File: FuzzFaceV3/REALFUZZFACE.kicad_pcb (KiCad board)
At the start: 2 copper layers, 48.5 x 35.2 mm, 22 parts, among them Q1 2SA1015, Q2 2SA1015

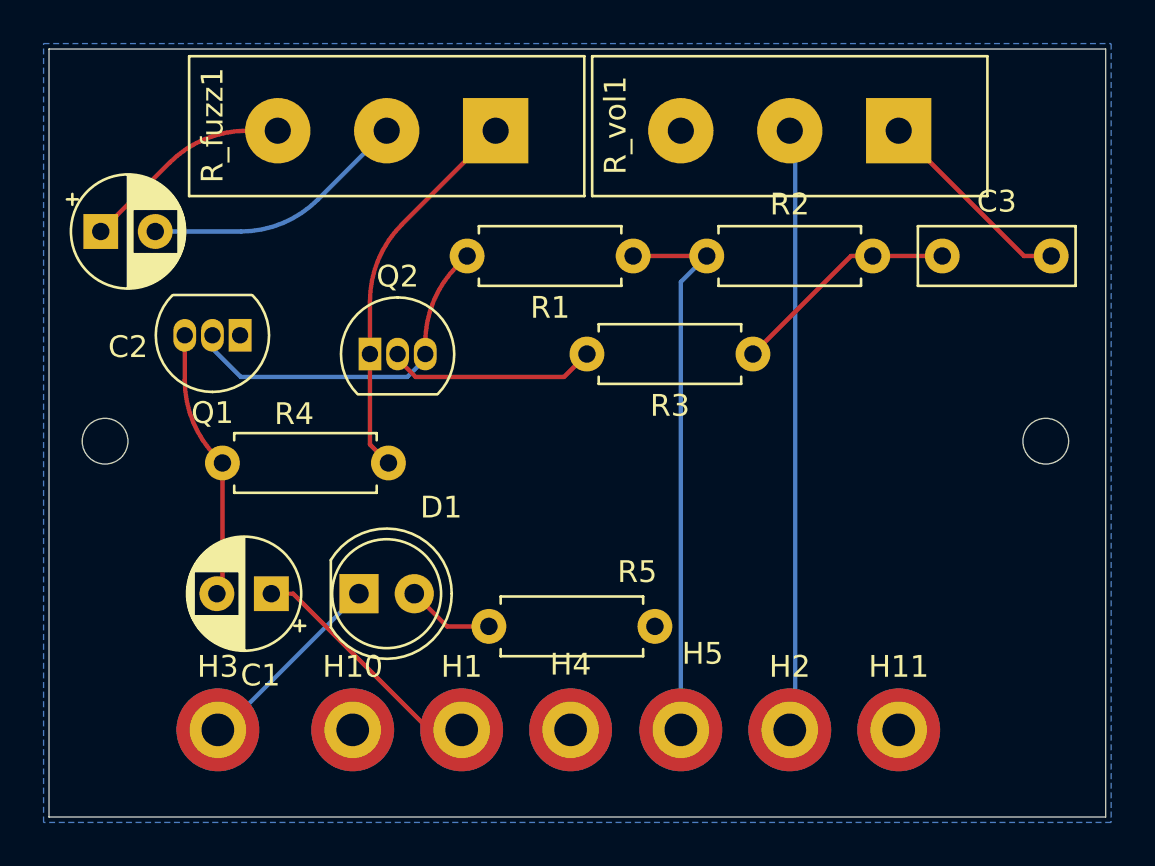
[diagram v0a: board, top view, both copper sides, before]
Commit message: done
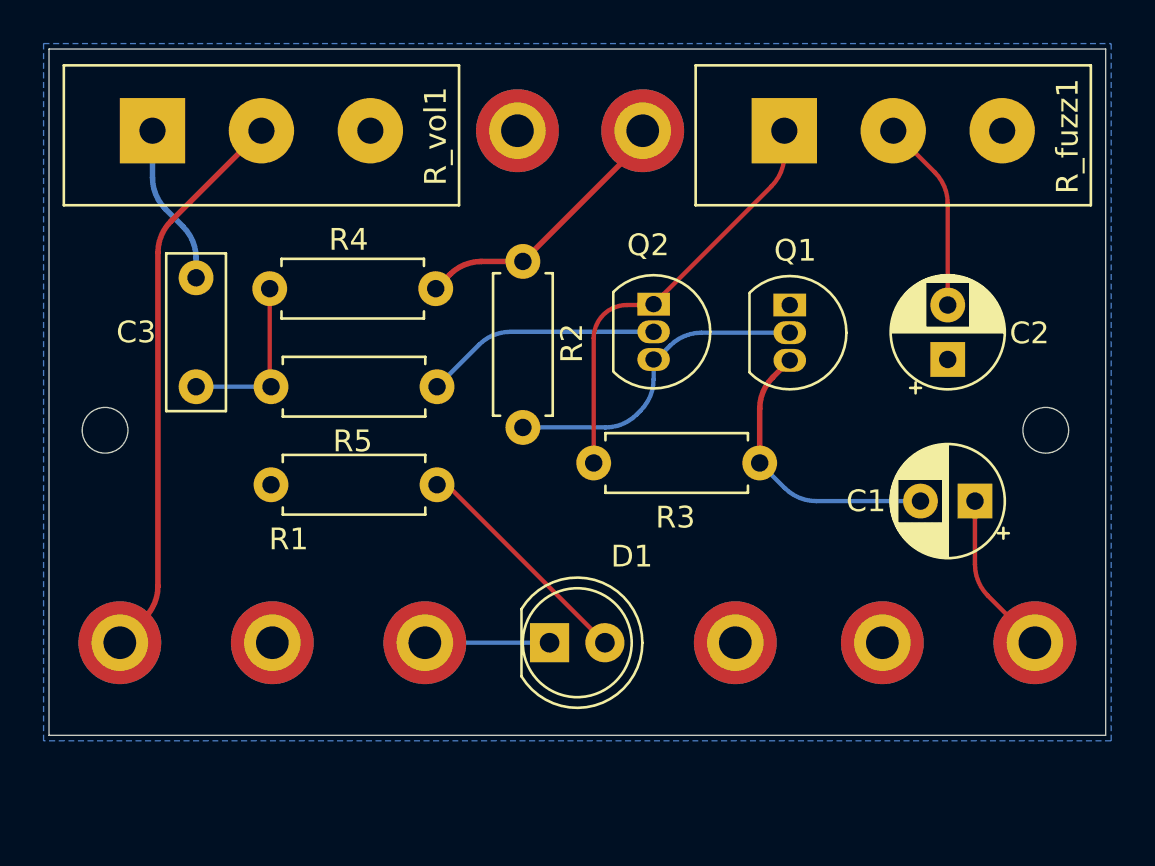
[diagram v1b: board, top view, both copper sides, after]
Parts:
- added P_GND1: P_GND, ANA PARTS:1.5mm_MountingHole, F.Cu at (153.8, 53.0)
- IN1: renamed from H1; value Input -> IN
- IN_GND1: renamed from H10; value In GND -> IN_GND
- MH1: renamed from H6; value MountingHole -> MH1
- MH2: renamed from H7; value MountingHole -> MH2
- OUT1: renamed from H2; value Output -> OUT
- OUT_GND1: renamed from H11; value Out GND -> OUT_GND
- PWR1: renamed from H5; value -9V -> PWR
- moved C2 39.3 mm to (173.5, 63.5), turned to 90 degrees
- moved C3 34.8 mm to (139.0, 64.8), turned to 90 degrees
- moved R_vol1 34.3 mm to (137.0, 52.5), turned to 90 degrees
- moved C1 32.6 mm to (174.8, 70.0)
- moved OUT1 31.0 mm to (135.5, 76.5)
- moved OUT_GND1 29.0 mm to (142.5, 76.5)
- moved PWR1 27.6 mm to (159.5, 53.0)
- moved IN1 26.6 mm to (177.5, 76.5)
- moved Q1 25.3 mm to (166.2, 61.0), turned to -90 degrees
- moved R3 24.7 mm to (164.9, 68.2), turned to 180 degrees
- moved IN_GND1 24.6 mm to (170.5, 76.5)
- moved R5 22.2 mm to (142.4, 64.8), turned to 0 degrees
- moved R1 18.8 mm to (142.4, 69.2), turned to 0 degrees
- moved R_fuzz1 13.3 mm to (166.0, 52.5), turned to 90 degrees
- moved Q2 13.2 mm to (160.0, 61.0), turned to -90 degrees
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- renumbered H4 to GND1, R5 to R1, R1 to R2, R4 to R3, R2 to R4, R3 to R5, H3 to SW1
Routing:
- net Net-(PWR1-Pad1): track 25.6 -> 12.7 mm
- net GND: track 10.2 -> 0.00 mm
- net Net-(D1-A): track 4.05 -> 10.7 mm
- net Net-(C1-Pad1): track 11.3 -> 7.54 mm
- net Net-(C2-Pad2): track 12.3 -> 8.94 mm
- net Net-(D1-K): track 9.06 -> 5.72 mm
- net Net-(C3-Pad1): track 10.6 -> 7.96 mm
- net Net-(C3-Pad2): track 9.38 -> 7.38 mm
- net Net-(Q2-E): track 17.8 -> 19.6 mm
- net Net-(Q1-C): track 16.5 -> 14.8 mm
- net Net-(OUT1-Pad1): track 27.6 -> 26.0 mm
- net Net-(Q2-C): track 9.69 -> 10.9 mm
- net Net-(Q1-B): track 12.4 -> 13.2 mm
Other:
- board size 48.5 x 35.2 mm -> 48.5 x 31.5 mm
